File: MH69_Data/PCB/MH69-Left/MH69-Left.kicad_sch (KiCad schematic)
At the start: 79 parts, among them J1 OLED/E-Ink_L, U1 nice_nano

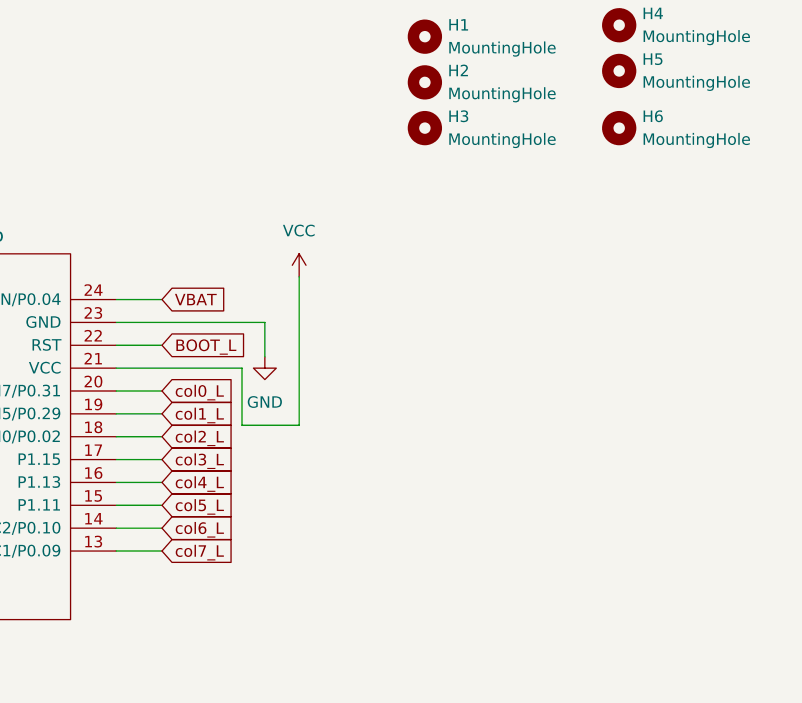
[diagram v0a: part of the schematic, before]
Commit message: Left side finished?
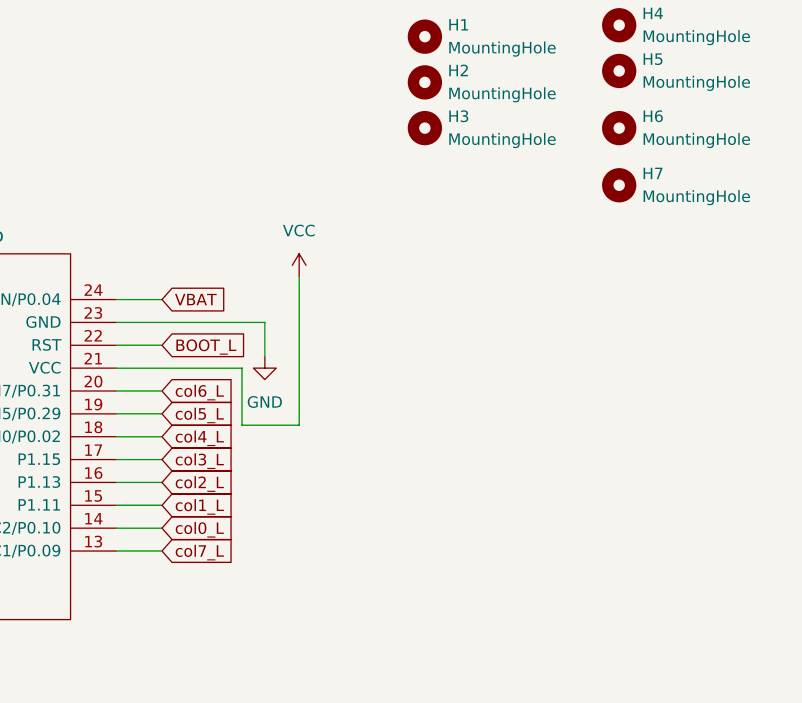
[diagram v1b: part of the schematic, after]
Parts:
- added H7: MountingHole, ScottoKeebs_Scotto:Standoff_M2x6mm, symbol Mechanical:MountingHole
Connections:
- net col0_L: now also U1.14 (NFC2/P0.10); no longer U1.20 (AIN7/P0.31)
- net col1_L: now also U1.15 (P1.11); no longer U1.19 (AIN5/P0.29)
- net col2_L: now also U1.16 (P1.13); no longer U1.18 (AIN0/P0.02)
- net col4_L: now also U1.18 (AIN0/P0.02); no longer U1.16 (P1.13)
- net col5_L: now also U1.19 (AIN5/P0.29); no longer U1.15 (P1.11)
- net col6_L: now also U1.20 (AIN7/P0.31); no longer U1.14 (NFC2/P0.10)
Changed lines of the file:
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@@
 	(wire
 		(pts
-			(xy 298.45 73.66) (xy 303.53 73.66)
-		)
-		(stroke
-			(width 0)
-			(type default)
-		)
-	)
-	(wire
-		(pts
 			(xy 191.77 74.93) (xy 198.12 74.93)
 		)
@@
 	(wire
 		(pts
-			(xy 298.45 81.28) (xy 303.53 81.28)
-		)
-		(stroke
-			(width 0)
-			(type default)
-		)
-	)
-	(wire
-		(pts
 			(xy 298.45 60.96) (xy 303.53 60.96)
 		)
@@
 	(wire
 		(pts
-			(xy 298.45 78.74) (xy 303.53 78.74)
+			(xy 34.29 111.76) (xy 85.09 111.76)
 		)
 		(stroke
@@
 	(wire
 		(pts
-			(xy 298.45 71.12) (xy 303.53 71.12)
+			(xy 298.45 83.82) (xy 303.53 83.82)
 		)
 		(stroke
@@
 	(wire
 		(pts
-			(xy 34.29 111.76) (xy 85.09 111.76)
+			(xy 161.29 105.41) (xy 161.29 106.68)
 		)
 		(stroke
@@
 	(wire
 		(pts
-			(xy 161.29 105.41) (xy 161.29 106.68)
+			(xy 191.77 24.13) (xy 198.12 24.13)
 		)
 		(stroke
@@
 	(wire
 		(pts
-			(xy 191.77 24.13) (xy 198.12 24.13)
+			(xy 298.45 55.88) (xy 303.53 55.88)
 		)
 		(stroke
@@
 	(wire
 		(pts
-			(xy 298.45 55.88) (xy 303.53 55.88)
+			(xy 110.49 60.96) (xy 135.89 60.96)
 		)
 		(stroke
@@
 	(wire
 		(pts
-			(xy 110.49 60.96) (xy 135.89 60.96)
+			(xy 262.89 60.96) (xy 248.92 60.96)
 		)
 		(stroke
@@
 	(wire
 		(pts
-			(xy 262.89 60.96) (xy 248.92 60.96)
+			(xy 172.72 16.51) (xy 172.72 24.13)
 		)
 		(stroke
@@
 	(wire
 		(pts
-			(xy 172.72 16.51) (xy 172.72 24.13)
+			(xy 298.45 71.12) (xy 303.53 71.12)
 		)
 		(stroke
@@
 	(wire
 		(pts
-			(xy 298.45 68.58) (xy 303.53 68.58)
+			(xy 246.38 16.51) (xy 246.38 24.13)
 		)
 		(stroke
@@
 	(wire
 		(pts
-			(xy 246.38 16.51) (xy 246.38 24.13)
+			(xy 298.45 66.04) (xy 303.53 66.04)
 		)
 		(stroke
@@
 	(wire
 		(pts
-			(xy 298.45 76.2) (xy 303.53 76.2)
-		)
-		(stroke
-			(width 0)
-			(type default)
-		)
-	)
-	(wire
-		(pts
 			(xy 212.09 35.56) (xy 237.49 35.56)
 		)
@@
 	(wire
 		(pts
+			(xy 298.45 73.66) (xy 303.53 73.66)
+		)
+		(stroke
+			(width 0)
+			(type default)
+		)
+	)
+	(wire
+		(pts
 			(xy 115.57 49.53) (xy 121.92 49.53)
 		)
@@
 	(wire
 		(pts
+			(xy 298.45 68.58) (xy 303.53 68.58)
+		)
+		(stroke
+			(width 0)
+			(type default)
+		)
+	)
+	(wire
+		(pts
 			(xy 96.52 74.93) (xy 96.52 49.53)
 		)
@@
 	(wire
 		(pts
+			(xy 298.45 76.2) (xy 303.53 76.2)
+		)
+		(stroke
+			(width 0)
+			(type default)
+		)
+	)
+	(wire
+		(pts
 			(xy 161.29 130.81) (xy 161.29 132.08)
 		)
@@
 	(wire
 		(pts
-			(xy 298.45 83.82) (xy 303.53 83.82)
-		)
-		(stroke
-			(width 0)
-			(type default)
-		)
-	)
-	(wire
-		(pts
 			(xy 161.29 137.16) (xy 186.69 137.16)
 		)
@@
 	(wire
 		(pts
+			(xy 298.45 78.74) (xy 303.53 78.74)
+		)
+		(stroke
+			(width 0)
+			(type default)
+		)
+	)
+	(wire
+		(pts
 			(xy 260.35 81.28) (xy 262.89 81.28)
 		)
@@
 	(wire
 		(pts
-			(xy 110.49 29.21) (xy 110.49 30.48)
+			(xy 298.45 81.28) (xy 303.53 81.28)
 		)
 		(stroke
@@
 	(wire
 		(pts
-			(xy 298.45 66.04) (xy 303.53 66.04)
+			(xy 110.49 29.21) (xy 110.49 30.48)
 		)
 		(stroke
@@
 	(global_label "col2_L"
 		(shape input)
-		(at 303.53 71.12 0)
+		(at 303.53 76.2 0)
 		(effects
 			(font
@@
 		)
 		(property "Intersheetrefs" "${INTERSHEET_REFS}"
-			(at 303.53 71.12 0)
+			(at 303.53 76.2 0)
 			(effects
 				(font
@@
 	(global_label "col6_L"
 		(shape input)
-		(at 303.53 81.28 0)
+		(at 303.53 66.04 0)
 		(effects
 			(font
@@
 		)
 		(property "Intersheetrefs" "${INTERSHEET_REFS}"
-			(at 303.53 81.28 0)
+			(at 303.53 66.04 0)
 			(effects
 				(font
@@
 	(global_label "col1_L"
 		(shape input)
-		(at 303.53 68.58 0)
+		(at 303.53 78.74 0)
 		(effects
 			(font
@@
 		)
 		(property "Intersheetrefs" "${INTERSHEET_REFS}"
-			(at 303.53 68.58 0)
+			(at 303.53 78.74 0)
 			(effects
 				(font
@@
 	(global_label "col4_L"
 		(shape input)
-		(at 303.53 76.2 0)
+		(at 303.53 71.12 0)
 		(effects
 			(font
@@
 		)
 		(property "Intersheetrefs" "${INTERSHEET_REFS}"
-			(at 303.53 76.2 0)
+			(at 303.53 71.12 0)
 			(effects
 				(font
@@
 	(global_label "col5_L"
 		(shape input)
-		(at 303.53 78.74 0)
+		(at 303.53 68.58 0)
 		(effects
 			(font
@@
 		)
 		(property "Intersheetrefs" "${INTERSHEET_REFS}"
-			(at 303.53 78.74 0)
+			(at 303.53 68.58 0)
 			(effects
 				(font
@@
 	(global_label "col0_L"
 		(shape input)
-		(at 303.53 66.04 0)
+		(at 303.53 81.28 0)
 		(effects
 			(font
@@
 		)
 		(property "Intersheetrefs" "${INTERSHEET_REFS}"
-			(at 303.53 66.04 0)
+			(at 303.53 81.28 0)
 			(effects
 				(font
@@
 					(unit 1)
 				)
+			)
+		)
+	)
+	(symbol
+		(lib_id "Mechanical:MountingHole")
+		(at 354.33 43.18 0)
+		(unit 1)
+		(exclude_from_sim yes)
+		(in_bom no)
+		(on_board yes)
+		(dnp no)
+		(fields_autoplaced yes)
+		(property "Reference" "H7"
+			(at 356.87 41.9099 0)
+			(effects
+				(font
+					(size 1.27 1.27)
+				)
+				(justify left)
+			)
+		)
+		(property "Value" "MountingHole"
+			(at 356.87 44.4499 0)
+			(effects
+				(font
+					(size 1.27 1.27)
+				)
+				(justify left)
+			)
+		)
+		(property "Footprint" "ScottoKeebs_Scotto:Standoff_M2x6mm"
+			(at 354.33 43.18 0)
+			(effects
+				(font
+					(size 1.27 1.27)
+				)
+				(hide yes)
+			)
+		)
+		(property "Datasheet" "~"
+			(at 354.33 43.18 0)
+			(effects
+				(font
+					(size 1.27 1.27)
+				)
+				(hide yes)
+			)
+		)
+		(property "Description" "Mounting Hole without connection"
+			(at 354.33 43.18 0)
+			(effects
+				(font
+					(size 1.27 1.27)
+				)
+				(hide yes)
+			)
+		)
+		(instances
+			(project "MH69-Left"
+				(path "/ea7de392-007d-439a-bcfc-3322a1a7900b"
+					(reference "H7")
+					(unit 1)
+				)
